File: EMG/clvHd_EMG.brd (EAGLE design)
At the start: 25 x 20 mm, 23 parts, among them J1 XF2J-1024-12, J2 XF2J-1024-12, U1 ADS1293CISQ/NOPB, X1 BM02B-SRSS-TB

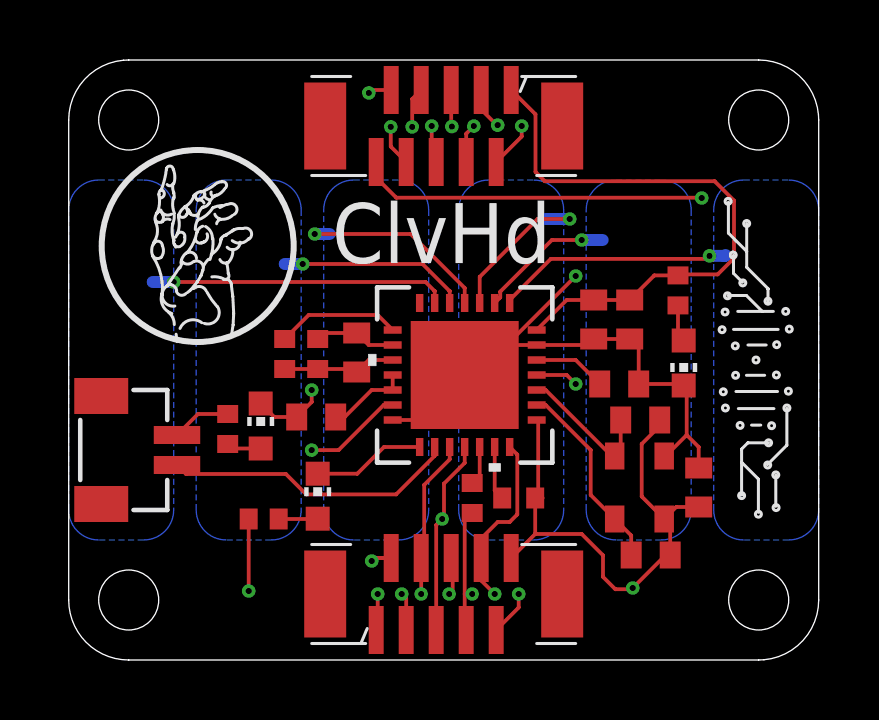
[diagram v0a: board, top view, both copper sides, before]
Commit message: update
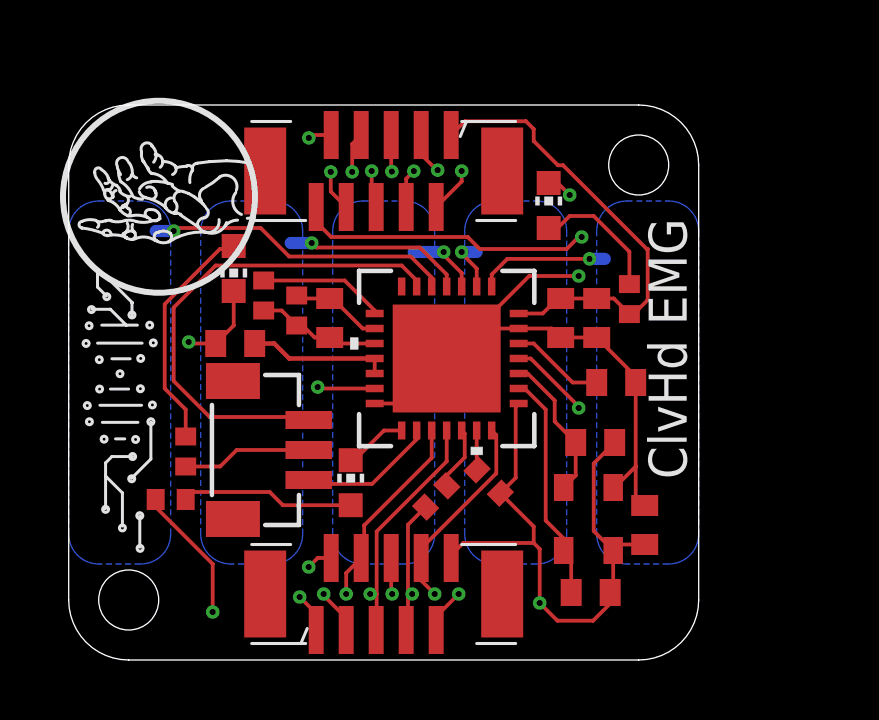
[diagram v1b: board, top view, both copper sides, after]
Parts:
- X1: value BM02B-SRSS-TB -> BM03B-SRSS-TB; device con-JST SH:BM02B-SRSS-TB -> con-JST SH:BM03B-SRSS-TB
- moved L1 6.91 mm to (16.0, 15.2), turned to 0 degrees
- moved L3 5.33 mm to (5.50, 13.1), turned to 180 degrees
- moved X1 4.39 mm to (8.00, 7.00)
- moved C12 3.65 mm to (5.55, 10.6)
- moved R12 3.17 mm to (3.40, 5.35)
- moved J2 2.50 mm to (10.5, 16.3)
- moved C10 2.36 mm to (17.4, 2.25)
- moved C13 2.19 mm to (19.2, 4.50)
- moved R14 2.07 mm to (6.50, 12.2)
- moved J1 2.00 mm to (10.5, 2.20)
- moved U$1 2.00 mm to (17.3, 4.70)
- moved C9 1.68 mm to (17.6, 7.25)
- moved R7 1.65 mm to (18.7, 12.0), turned to 90 degrees
- moved R15 1.61 mm to (7.60, 11.7)
- moved R1 1.59 mm to (3.90, 6.95), turned to 270 degrees
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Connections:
- net IN2. renamed IN2
- net IN6: now also X1.3
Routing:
- net IN6: track 9.93 -> 16.6 mm, vias 1 -> 0
- net N$7: track 1.16 -> 7.80 mm
- net CS: track 9.82 -> 4.83 mm
- net N$6: track 1.30 -> 5.79 mm
- net SYNCB: track 22.5 -> 18.5 mm
- net IN5: track 6.28 -> 10.2 mm
- net IN1: track 7.92 -> 4.39 mm
- net N$2: track 1.25 -> 4.43 mm
- net IN3: track 5.47 -> 2.40 mm
- net IN2: track 4.58 -> 1.86 mm
- net N$5: track 1.98 -> 4.33 mm
- net DIN: track 21.1 -> 23.3 mm
- net RLDREF: track 2.77 -> 4.71 mm
- net GND: track 33.6 -> 35.3 mm, vias 8 -> 9
- net ALARMB: track 3.77 -> 2.11 mm
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- removed copper zone on layer 16, net IN6
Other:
- board size 25 x 20 mm -> 21 x 18.5 mm
- board text added: "ClvHd EMG"
- board text added: "ads1293-4l-fpc-v12"
- board text removed: "2"
- board text removed: "3"
- board text removed: "4"
- board text removed: "6"
- board text removed: "ClvHd"
- board text removed: "ads1293-4l-fpc-v10"
